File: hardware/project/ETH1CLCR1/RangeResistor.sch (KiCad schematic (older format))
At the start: 109 parts, among them K801 TQ2SA-5V, Q801 BC847W, Q802 2N2218A, Q803 2N2904A, Q804 BC847W, Q805 BC847W, Q806 BC847W, Q807 BC847W, Q808 BC847W, U801 AD5293BRUZ-20, U802 TL072, U803 AQY212GS, U804 HA3-2525-5Z, U805 AQY212GS, U806 AQY212GS, U807 AQY212GS, U808 AQY212GS, U809 AQY212GS, U810 AQY212GS, U811 AQY212GS, U812 AQY212GS, U813 AQY212GS, U814 AQY212GS, U815 AQY212GS

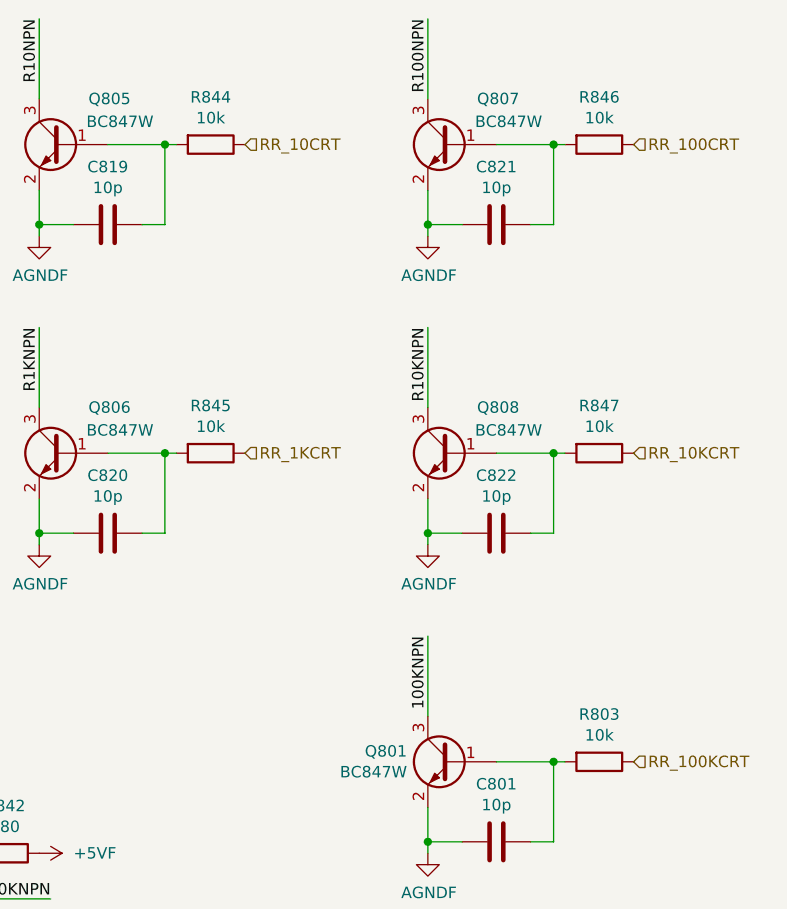
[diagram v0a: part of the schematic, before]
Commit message: Range BC847 base serial resistors value from 10k to 1k.
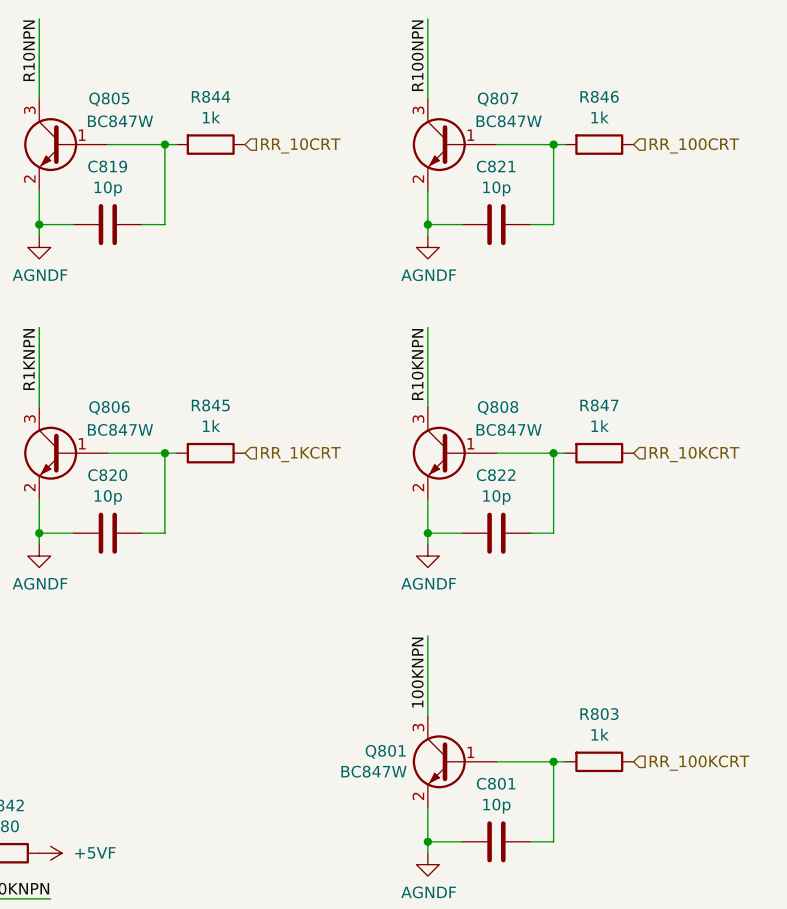
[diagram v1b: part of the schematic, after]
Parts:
- R803, R844, R845, R846, R847: value 10k -> 1k
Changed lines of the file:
@@
 P 15150 3900
 F 0 "R803" V 14943 3900 50  0000 C CNN
-F 1 "10k" V 15034 3900 50  0000 C CNN
+F 1 "1k" V 15034 3900 50  0000 C CNN
 F 2 "Resistor_SMD:R_0603_1608Metric_Pad1.05x0.95mm_HandSolder" V 15080 3900 50  0001 C CNN
 F 3 "~" H 15150 3900 50  0001 C CNN
@@
 P 13450 1200
 F 0 "R844" V 13243 1200 50  0000 C CNN
-F 1 "10k" V 13334 1200 50  0000 C CNN
+F 1 "1k" V 13334 1200 50  0000 C CNN
 F 2 "Resistor_SMD:R_0603_1608Metric_Pad1.05x0.95mm_HandSolder" V 13380 1200 50  0001 C CNN
 F 3 "~" H 13450 1200 50  0001 C CNN
@@
 P 15150 1200
 F 0 "R846" V 14943 1200 50  0000 C CNN
-F 1 "10k" V 15034 1200 50  0000 C CNN
+F 1 "1k" V 15034 1200 50  0000 C CNN
 F 2 "Resistor_SMD:R_0603_1608Metric_Pad1.05x0.95mm_HandSolder" V 15080 1200 50  0001 C CNN
 F 3 "~" H 15150 1200 50  0001 C CNN
@@
 P 13450 2550
 F 0 "R845" V 13243 2550 50  0000 C CNN
-F 1 "10k" V 13334 2550 50  0000 C CNN
+F 1 "1k" V 13334 2550 50  0000 C CNN
 F 2 "Resistor_SMD:R_0603_1608Metric_Pad1.05x0.95mm_HandSolder" V 13380 2550 50  0001 C CNN
 F 3 "~" H 13450 2550 50  0001 C CNN
@@
 P 15150 2550
 F 0 "R847" V 14943 2550 50  0000 C CNN
-F 1 "10k" V 15034 2550 50  0000 C CNN
+F 1 "1k" V 15034 2550 50  0000 C CNN
 F 2 "Resistor_SMD:R_0603_1608Metric_Pad1.05x0.95mm_HandSolder" V 15080 2550 50  0001 C CNN
 F 3 "~" H 15150 2550 50  0001 C CNN

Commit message: Changed BC847W base resistor from 1k to 10k.
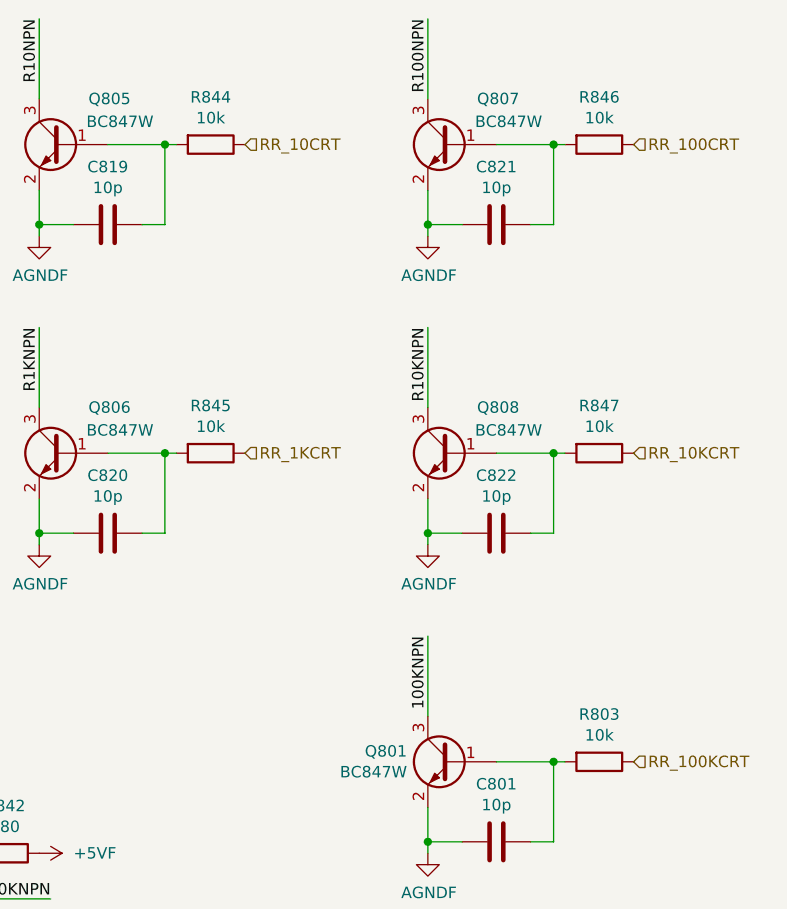
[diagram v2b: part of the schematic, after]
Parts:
- R803, R844, R845, R846, R847: value 1k -> 10k
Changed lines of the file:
@@
 P 15150 3900
 F 0 "R803" V 14943 3900 50  0000 C CNN
-F 1 "1k" V 15034 3900 50  0000 C CNN
+F 1 "10k" V 15034 3900 50  0000 C CNN
 F 2 "Resistor_SMD:R_0603_1608Metric_Pad1.05x0.95mm_HandSolder" V 15080 3900 50  0001 C CNN
 F 3 "~" H 15150 3900 50  0001 C CNN
@@
 P 13450 1200
 F 0 "R844" V 13243 1200 50  0000 C CNN
-F 1 "1k" V 13334 1200 50  0000 C CNN
+F 1 "10k" V 13334 1200 50  0000 C CNN
 F 2 "Resistor_SMD:R_0603_1608Metric_Pad1.05x0.95mm_HandSolder" V 13380 1200 50  0001 C CNN
 F 3 "~" H 13450 1200 50  0001 C CNN
@@
 P 15150 1200
 F 0 "R846" V 14943 1200 50  0000 C CNN
-F 1 "1k" V 15034 1200 50  0000 C CNN
+F 1 "10k" V 15034 1200 50  0000 C CNN
 F 2 "Resistor_SMD:R_0603_1608Metric_Pad1.05x0.95mm_HandSolder" V 15080 1200 50  0001 C CNN
 F 3 "~" H 15150 1200 50  0001 C CNN
@@
 P 13450 2550
 F 0 "R845" V 13243 2550 50  0000 C CNN
-F 1 "1k" V 13334 2550 50  0000 C CNN
+F 1 "10k" V 13334 2550 50  0000 C CNN
 F 2 "Resistor_SMD:R_0603_1608Metric_Pad1.05x0.95mm_HandSolder" V 13380 2550 50  0001 C CNN
 F 3 "~" H 13450 2550 50  0001 C CNN
@@
 P 15150 2550
 F 0 "R847" V 14943 2550 50  0000 C CNN
-F 1 "1k" V 15034 2550 50  0000 C CNN
+F 1 "10k" V 15034 2550 50  0000 C CNN
 F 2 "Resistor_SMD:R_0603_1608Metric_Pad1.05x0.95mm_HandSolder" V 15080 2550 50  0001 C CNN
 F 3 "~" H 15150 2550 50  0001 C CNN
